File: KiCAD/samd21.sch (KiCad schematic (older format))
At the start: 25 parts, among them J2 690-005-299-043, J3 Conn_01x03_Male, P9 SWD, U10 SN74AVC8T245PW, U7 MCP1700-3302E_SOT23, U8 ATSAMD21E18A-AF, U9 SN74AVC8T245PW, X1 ASE-xxxMHz

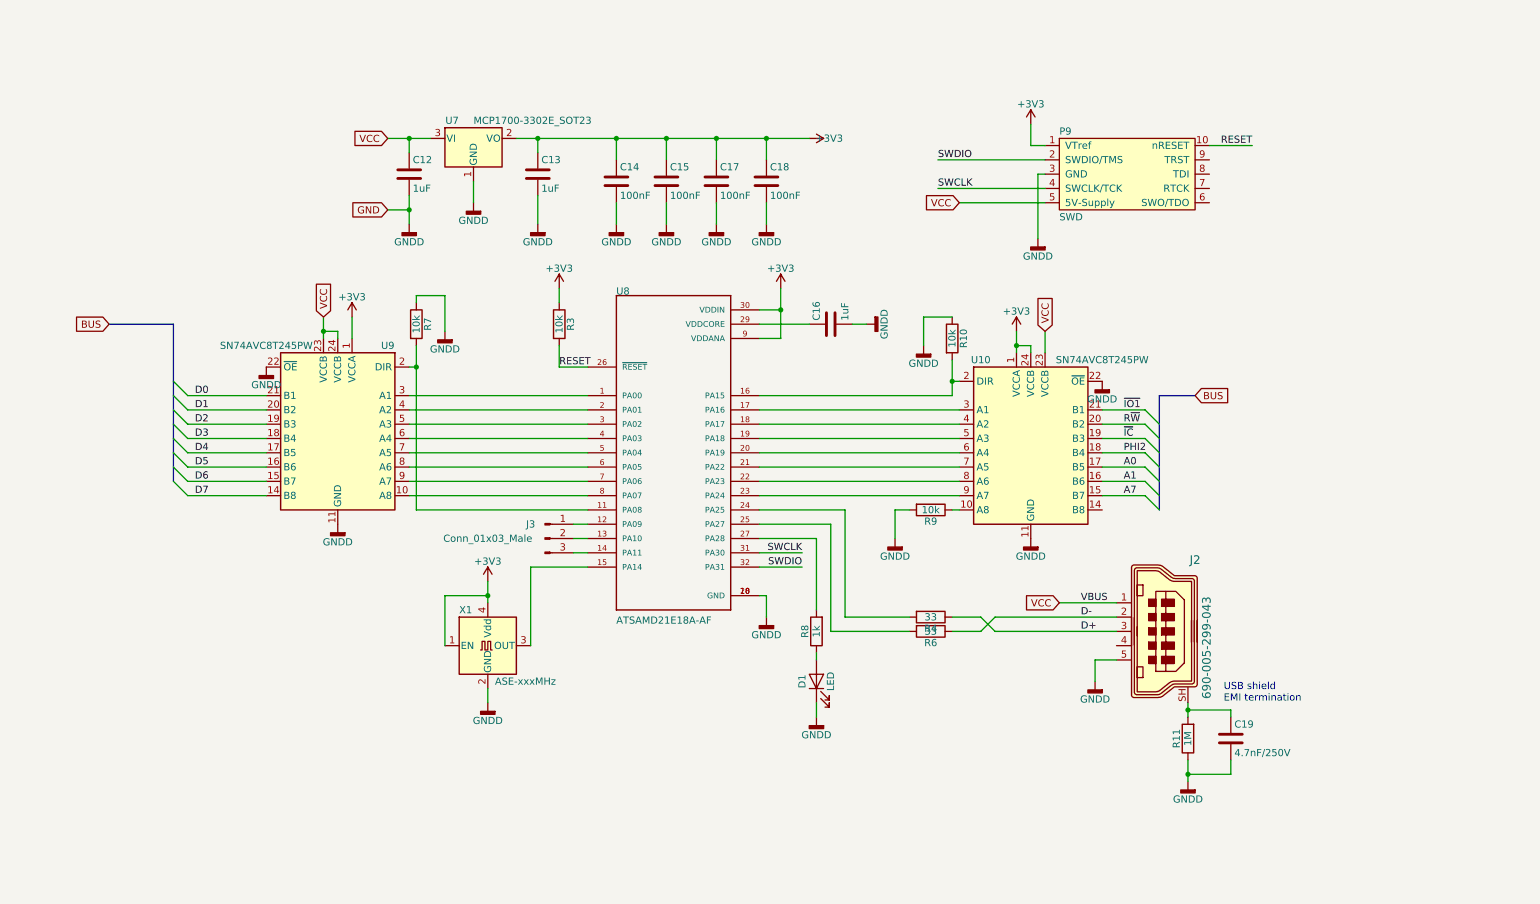
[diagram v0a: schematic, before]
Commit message: board routed
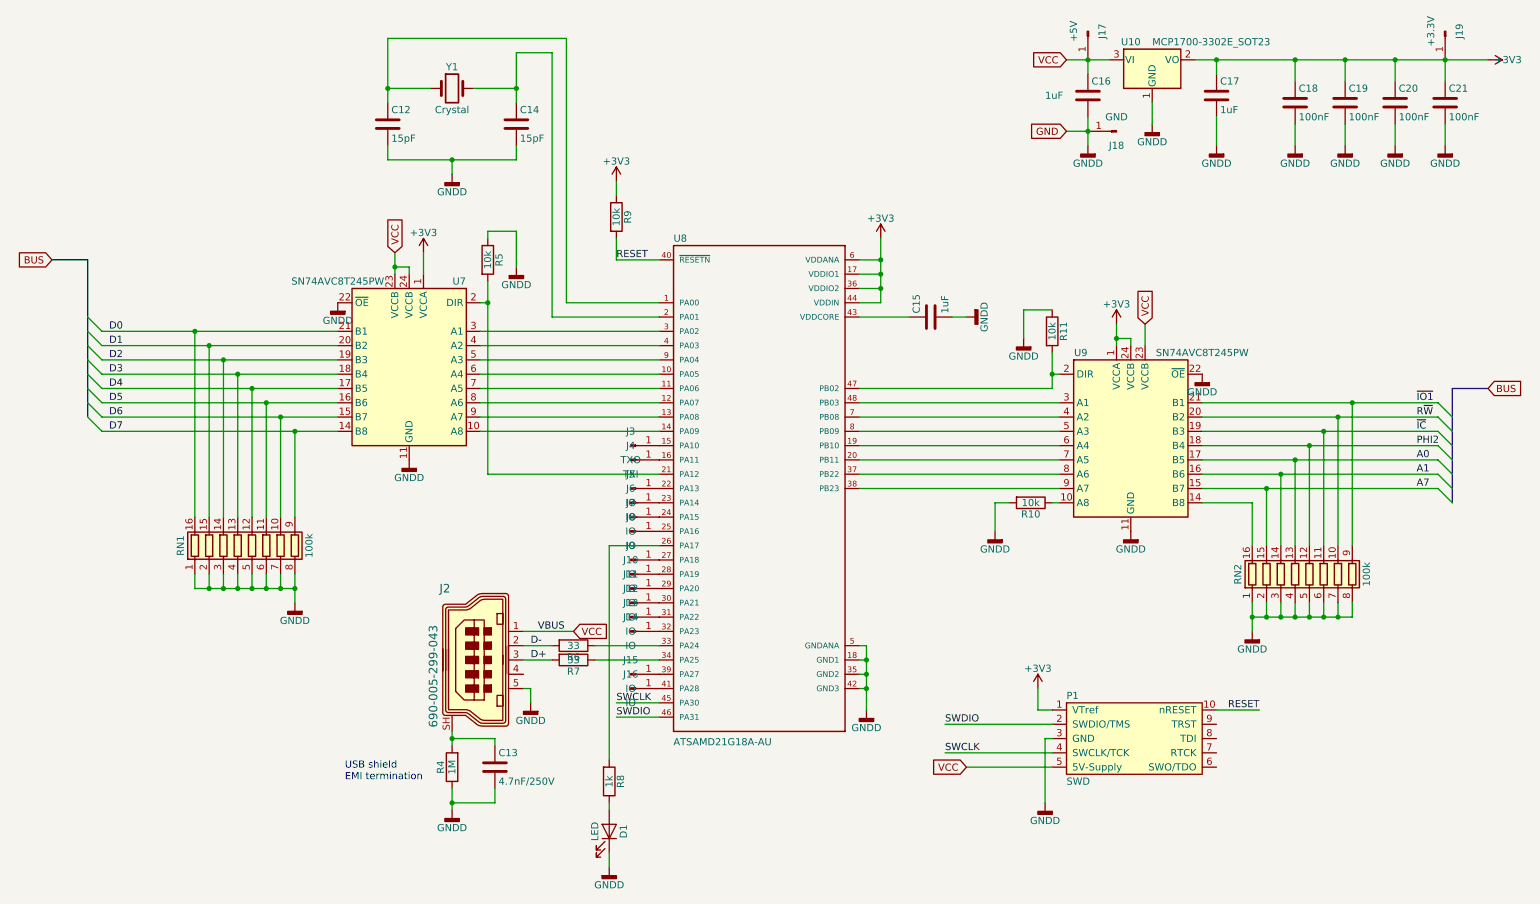
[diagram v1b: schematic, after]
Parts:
- removed J3: Conn_01x03_Male, Connector_PinHeader_2.54mm:PinHeader_1x03_P2.54mm_Vertical, symbol Connector:Conn_01x03_Male
- removed U8: ATSAMD21E18A-AF, ATSAMD21E18A-AF:QFP80P900X900X120-32N, symbol ATSAMD21E18A-AF:ATSAMD21E18A-AF
- removed X1: ASE-xxxMHz, Oscillator:Oscillator_SMD_Abracon_ASE-4Pin_3.2x2.5mm, symbol Oscillator:ASE-xxxMHz
- added C12, C14: 15pF, Capacitor_SMD:C_0805_2012Metric, symbol Device:C
- added J10, J11, J12, J13, J14, J15, J16, J5, J6, J7, J8, J9: IO, Connector_PinSocket_2.54mm:PinSocket_1x01_P2.54mm_Vertical, symbol Connector:Conn_01x01_Male
- added J17: +5V, Connector_PinSocket_2.54mm:PinSocket_1x01_P2.54mm_Vertical, symbol Connector:Conn_01x01_Male
- added J18: GND, Connector_PinSocket_2.54mm:PinSocket_1x01_P2.54mm_Vertical, symbol Connector:Conn_01x01_Male
- added J19: +3.3V, Connector_PinSocket_2.54mm:PinSocket_1x01_P2.54mm_Vertical, symbol Connector:Conn_01x01_Male
- added J3: TXO, Connector_PinSocket_2.54mm:PinSocket_1x01_P2.54mm_Vertical, symbol Connector:Conn_01x01_Male
- added J4: TXI, Connector_PinSocket_2.54mm:PinSocket_1x01_P2.54mm_Vertical, symbol Connector:Conn_01x01_Male
- added RN1, RN2: 100k, Resistor_SMD:R_Array_Convex_8x0602, symbol Device:R_Pack08
- added U8: ATSAMD21G18A-AU, ATSAMD21G18A-AU:QFP50P900X900X120-48N, symbol ATSAMD21G18A-AU:ATSAMD21G18A-AU
- added Y1: Crystal, Crystal:Crystal_SMD_3215-2Pin_3.2x1.5mm, symbol Device:Crystal
- renumbered C19 to C13, C16 to C15, C12 to C16, C13 to C17, C14 to C18, C15 to C19, C17 to C20, C18 to C21, P9 to P1, R9 to R10, R10 to R11, R11 to R4, R7 to R5, R4 to R6, R6 to R7, R3 to R9, U7 to U10, U9 to U7, U10 to U9
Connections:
- net +3V3: now also J19.1 (Pin_1), U8.17 (VDDIO1), U8.36 (VDDIO2), U8.44 (VDDIN), U8.6 (VDDANA)
- net A0: now also RN2.13 (R4.2)
- net A1: now also RN2.14 (R3.2)
- net A7: now also RN2.15 (R2.2)
- net D+: now also R7.2; no longer R6.1
- net D-: now also R6.2; no longer R7.1
- net D0: now also RN1.16 (R1.2)
- net D1: now also RN1.15 (R2.2)
- net D2: now also RN1.14 (R3.2)
- net D3: now also RN1.13 (R4.2)
- net D4: now also RN1.12 (R5.2)
- net D5: now also RN1.11 (R6.2)
- net D6: now also RN1.10 (R7.2)
- net D7: now also RN1.9 (R8.2)
- net GNDD: now also C12.2, C14.2, J18.1 (Pin_1), RN1.1 (R1.1), RN1.2 (R2.1), RN1.3 (R3.1), RN1.4 (R4.1), RN1.5 (R5.1), RN1.6 (R6.1), RN1.7 (R7.1), RN1.8 (R8.1), RN2.1 (R1.1), RN2.2 (R2.1), RN2.3 (R3.1), RN2.4 (R4.1), RN2.5 (R5.1), RN2.6 (R6.1), RN2.7 (R7.1), RN2.8 (R8.1), U8.18 (GND1), U8.35 (GND2), U8.42 (GND3), U8.5 (GNDANA)
- net PHI2: now also RN2.12 (R5.2)
- net RESET: now also U8.40 (~RESETN~)
- net R~W: now also RN2.10 (R7.2)
- net SWCLK: now also U8.45 (PA30)
- net SWDIO: now also U8.46 (PA31)
- net VCC: now also J17.1 (Pin_1)
- net ~IC: now also RN2.11 (R6.2)
- net ~IO1: now also RN2.9 (R8.2)
- net at U7.3 (A1): now also U8.3 (PA02)
- net at R5.2, U7.2 (DIR): now also U8.21 (PA12)
- net at R11.2, U9.2 (DIR): now also U8.47 (PB02)
- net at U9.3 (A1): now also U8.48 (PB03)
- net at U9.4 (A2): now also U8.7 (PB08)
- net at U9.5 (A3): now also U8.8 (PB09)
- net at U7.4 (A2): now also U8.4 (PA03)
- net at U9.6 (A4): now also U8.19 (PB10)
- net at U9.7 (A5): now also U8.20 (PB11)
- net at U9.8 (A6): now also U8.37 (PB22)
- net at U9.9 (A7): now also U8.38 (PB23)
- net at R8.2: now also U8.26 (PA17)
- net at C15.1: now also U8.43 (VDDCORE)
- net at U7.5 (A3): now also U8.9 (PA04)
- net at U7.6 (A4): now also U8.10 (PA05)
- net at U7.7 (A5): now also U8.11 (PA06)
- net at U7.8 (A6): now also U8.12 (PA07)
- net at U7.9 (A7): now also U8.13 (PA08)
- net at U7.10 (A8): now also U8.14 (PA09)
- net at U9.14 (B8): now also RN2.16 (R1.2)
- new net: C12.1, U8.1 (PA00), Y1.1
- new net: C14.1, U8.2 (PA01), Y1.2
- new net: J3.1 (Pin_1), U8.15 (PA10)
- new net: J4.1 (Pin_1), U8.16 (PA11)
- new net: J5.1 (Pin_1), U8.22 (PA13)
- new net: J6.1 (Pin_1), U8.23 (PA14)
- new net: J7.1 (Pin_1), U8.24 (PA15)
- new net: J8.1 (Pin_1), U8.25 (PA16)
- new net: J9.1 (Pin_1), U8.27 (PA18)
- new net: J10.1 (Pin_1), U8.28 (PA19)
- new net: J11.1 (Pin_1), U8.29 (PA20)
- new net: J12.1 (Pin_1), U8.30 (PA21)
- new net: J13.1 (Pin_1), U8.31 (PA22)
- new net: J14.1 (Pin_1), U8.32 (PA23)
- new net: R6.1, U8.33 (PA24)
- new net: R7.1, U8.34 (PA25)
- new net: J15.1 (Pin_1), U8.39 (PA27)
- new net: J16.1 (Pin_1), U8.41 (PA28)
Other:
- moved on the sheet: C13, C15, C16, C17, C18, C19, C20, C21, D1, J2, P1, R10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
